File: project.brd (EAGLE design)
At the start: 160 x 100 mm, 56 parts, among them Y1 ABM8-20.000MHZ-B2-T

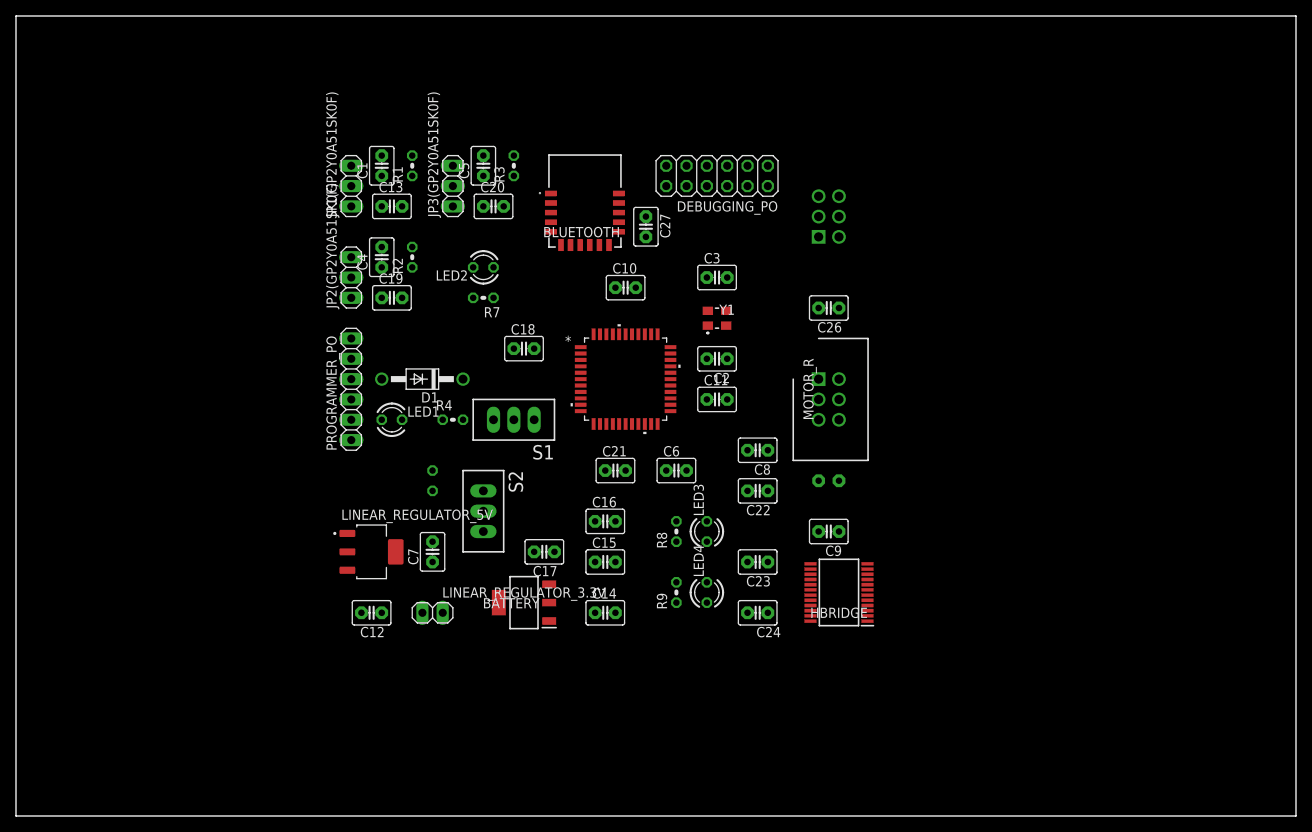
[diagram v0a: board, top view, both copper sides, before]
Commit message: route board
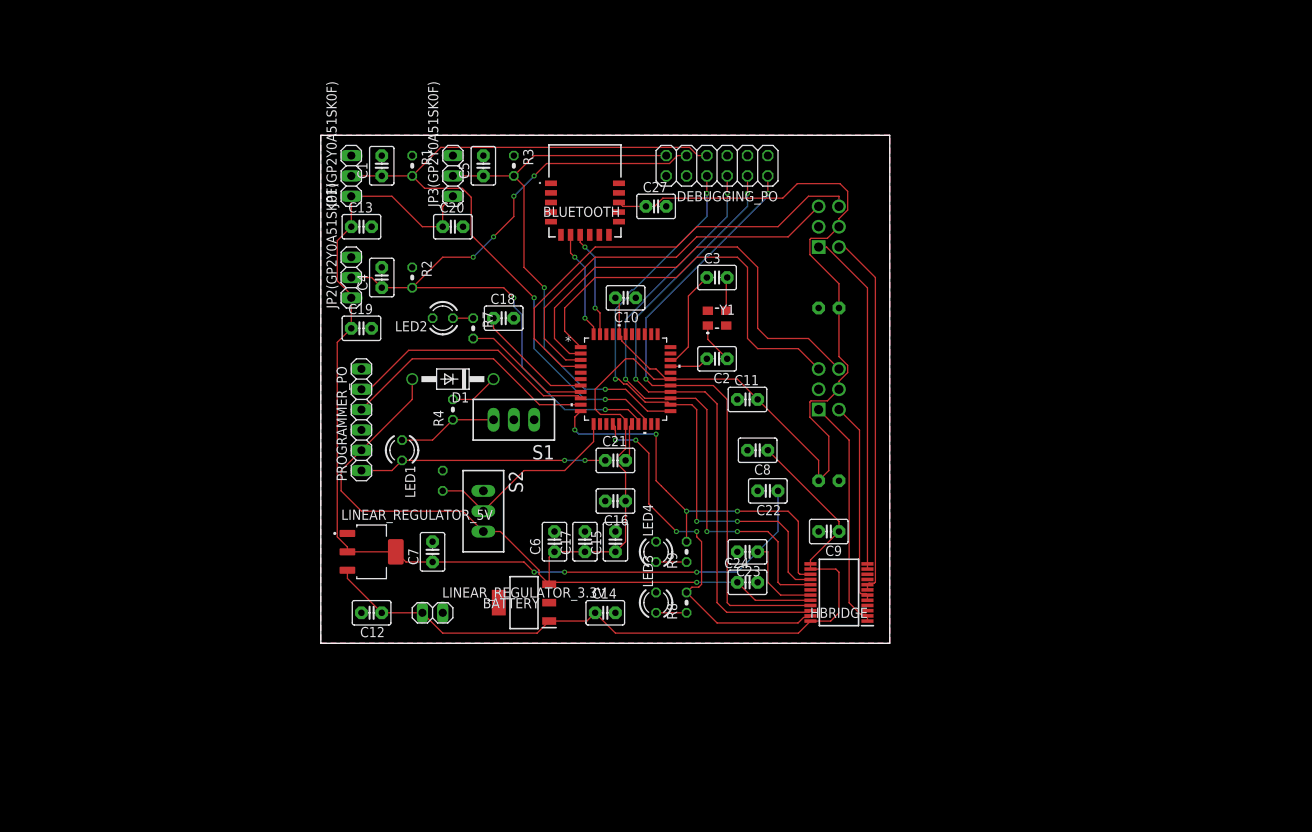
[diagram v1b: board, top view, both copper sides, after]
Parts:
- moved C25 21.6 mm to (101.6, 63.5)
- moved C26 21.6 mm to (101.6, 41.9), flipped to the bottom
- moved MOTOR_L 21.6 mm to (100.3, 50.8)
- moved C6 17.6 mm to (67.3, 34.3), turned to 90 degrees
- moved MOTOR_R 16.5 mm to (100.3, 71.1), flipped to the bottom, turned to 90 degrees
- moved LED3 10.9 mm to (80.0, 26.7)
- moved R8 8.98 mm to (83.8, 26.7)
- moved LED2 8.13 mm to (53.3, 62.2)
- moved LED4 8.13 mm to (80.0, 33.0)
- moved C20 5.68 mm to (54.6, 73.7)
- moved C19 5.39 mm to (43.2, 61.0)
- moved R9 5.24 mm to (83.8, 33.0)
- moved C17 5.24 mm to (71.1, 34.3), turned to 90 degrees
- moved C13 4.58 mm to (43.2, 73.7)
- moved C18 4.58 mm to (61.0, 62.2)
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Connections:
- removed net B01: HBRIDGE.12
- removed net PMW_L: DEBUGGING_PO.1, MICROCHIP.15
- removed net PMW_R: MICROCHIP.11
- net AN0: now also MICROCHIP.20; no longer MICROCHIP.19
- net AN1: now also MICROCHIP.19; no longer MICROCHIP.20
- net BO1: now also HBRIDGE.11, HBRIDGE.12
- net ENCL_A: now also MICROCHIP.1; no longer MICROCHIP.2
- net ENCL_B: now also MICROCHIP.2; no longer MICROCHIP.1
- net N$16: now also MICROCHIP.12; no longer MICROCHIP.43
- net PGEC1: now also MICROCHIP.9; no longer MICROCHIP.22
- net PGED1: now also MICROCHIP.10; no longer MICROCHIP.21
- net PWM_L: now also MICROCHIP.15
- net PWM_R: now also MICROCHIP.11; no longer DEBUGGING_PO.3
- net RX: now also MICROCHIP.44; no longer MICROCHIP.38
- net TX: now also MICROCHIP.43; no longer MICROCHIP.37
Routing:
- net 3.3V: track 0.00 -> 246.0 mm, vias 0 -> 1
- net 5V: track 0.00 -> 137.6 mm, vias 0 -> 3
- net VM: track 0.00 -> 97.3 mm
- net AN0: track 0.00 -> 95.3 mm, vias 0 -> 2
- net AN1: track 0.00 -> 90.9 mm, vias 0 -> 6
- net MTRDRV_AIN2: track 0.00 -> 79.7 mm, vias 0 -> 2
- net MTRDRV_AIN1: track 0.00 -> 78.9 mm, vias 0 -> 2
- net MTRDRV_BIN1: track 0.00 -> 76.3 mm, vias 0 -> 4
- net MTRDRV_BIN2: track 0.00 -> 76.2 mm, vias 0 -> 4
- net AN4: track 0.00 -> 69.9 mm, vias 0 -> 2
- net ENCL_B: track 0.00 -> 57.4 mm
- net ENCR_B: track 0.00 -> 56.2 mm
- net ENCL_A: track 0.00 -> 51.1 mm
- net PWM_R: track 0.00 -> 50.6 mm, vias 0 -> 4
- net ENCR_A: track 0.00 -> 49.0 mm
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- added copper zone on layer 1, net GND
- added copper zone on layer 16, net GND
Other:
- board size 160 x 100 mm -> 71.1 x 63.5 mm
